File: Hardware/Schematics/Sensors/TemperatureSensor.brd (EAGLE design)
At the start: 13.9 x 21.3 mm, 6 parts, among them IC1 DS18B20

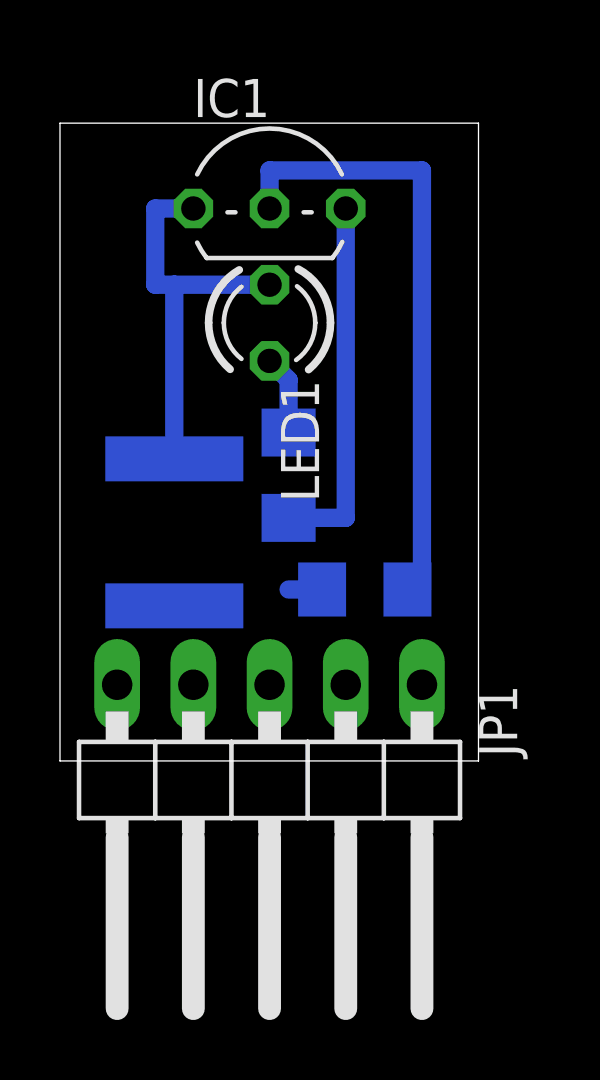
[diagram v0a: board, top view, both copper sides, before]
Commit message: sensors
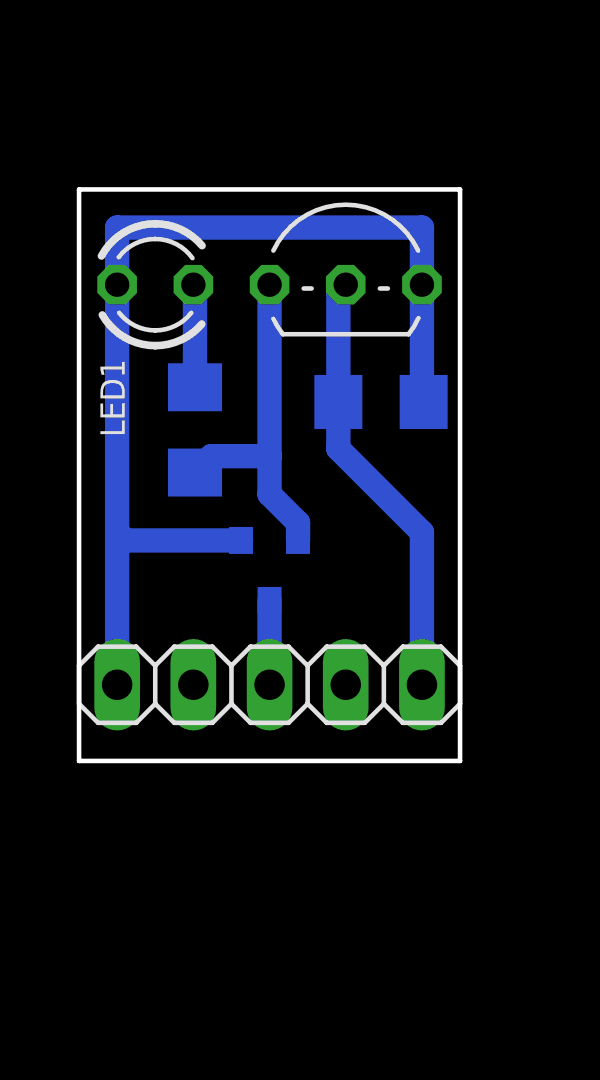
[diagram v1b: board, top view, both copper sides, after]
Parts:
- removed F1: 50ma, fuse:MF-SMDF050
- added Q1: BSS138, Cing Library:SOT23
- JP1: device pinhead:1X05/90 -> pinhead:1X05
- R1: value 4k7 -> 1k
- R2: value 1k -> 330
- moved R1 6.27 mm to (10.1, 12.0), turned to 0 degrees
- moved LED1 4.02 mm to (2.54, 15.9), turned to 0 degrees
- moved JP1 3.81 mm to (6.35, 2.54)
- moved IC1 3.59 mm to (8.89, 15.9)
- moved R2 3.47 mm to (3.87, 11.0)
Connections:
- removed net N$14: IC1.3, JP1.3, R1.1, R2.1
- removed net N$15: F1.1, JP1.5
- new net N$3: JP1.3, Q1.3
- new net N$4: IC1.1, Q1.2, R2.1
- net N$1: now also IC1.3, JP1.5, Q1.1, R1.1; no longer F1.2, IC1.1
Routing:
- net N$1: track 13.4 -> 35.5 mm
- net N$14: track 13.3 -> 0.00 mm
- net N$4: track 0.00 -> 11.6 mm
- net N$5: track 20.8 -> 14.6 mm
- net N$3: track 0.00 -> 2.81 mm
- net N$15: track 1.27 -> 0.00 mm
- net N$2: track 2.65 -> 3.44 mm
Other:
- board size 13.9 x 21.3 mm -> 12.7 x 19.1 mm
